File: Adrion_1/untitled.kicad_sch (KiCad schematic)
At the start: 3 parts, among them J6 M20-7821546, J7 M20-7821546, U6 NUCLEO-G431KB

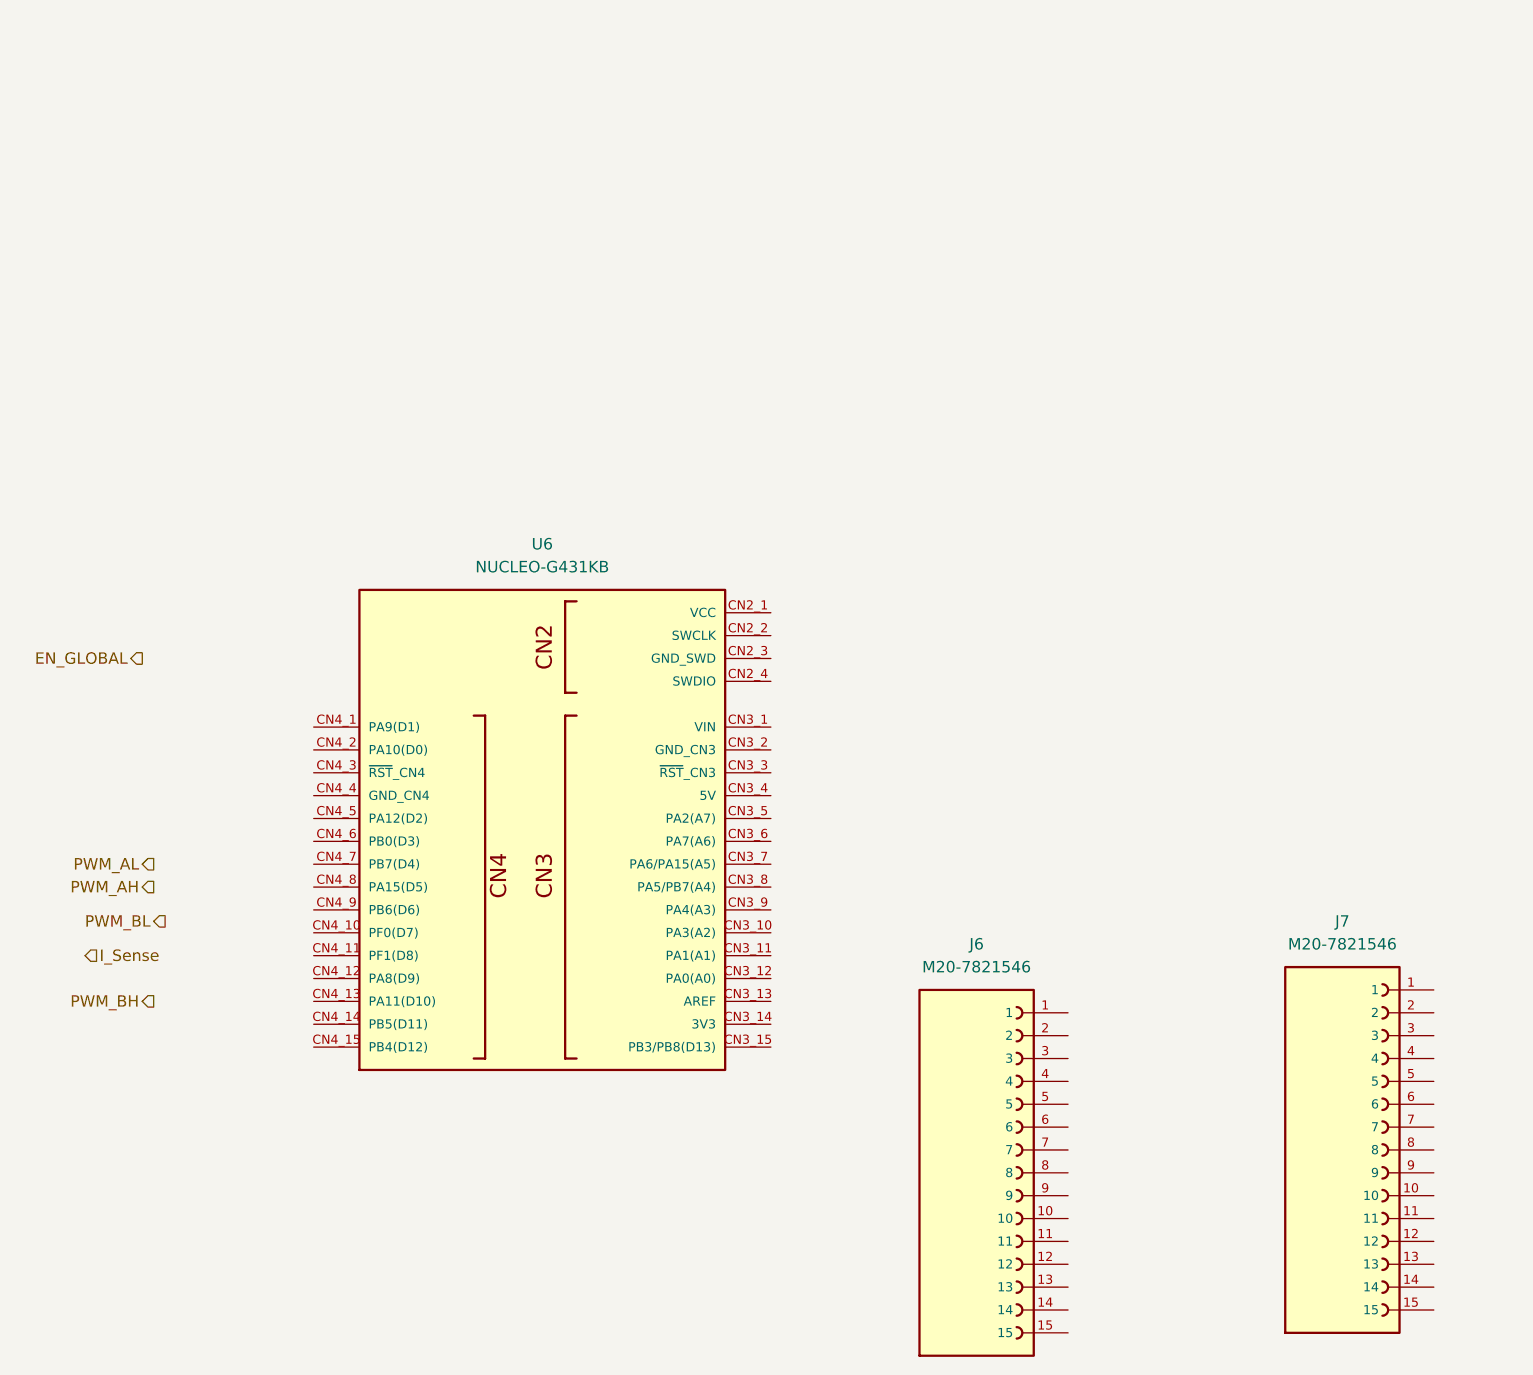
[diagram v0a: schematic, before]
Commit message: Mamita he empezado el layout. Vaya show
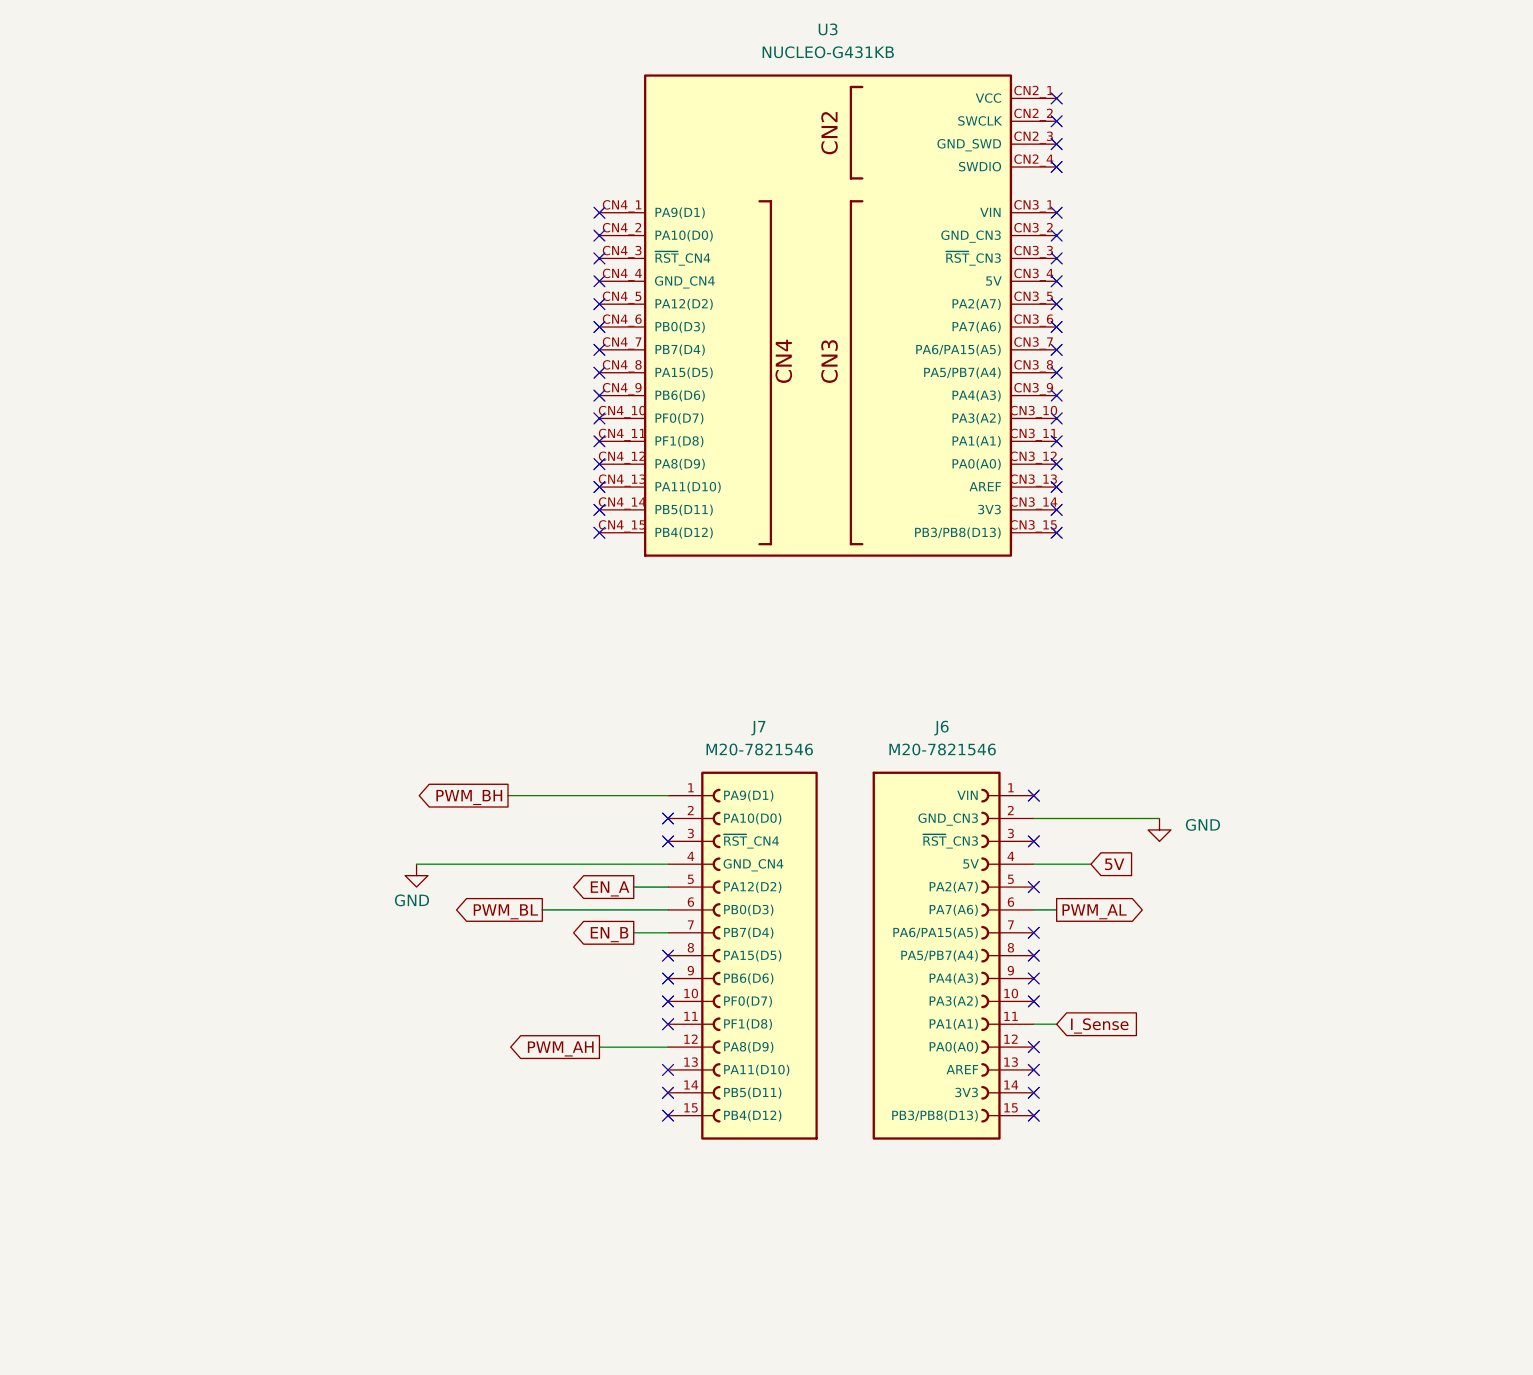
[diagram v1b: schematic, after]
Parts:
- removed U6: NUCLEO-G431KB, NUCLEO-G431KB:MODULE_NUCLEO-G431KB, symbol NUCLEO-G431KB:NUCLEO-G431KB
- added U3: NUCLEO-G431KB, MODULE_NUCLEO-G431KB:MODULE_NUCLEO-G431KB, symbol NUCLEO-G431KB:NUCLEO-G431KB
- J6, J7: footprint M20-7821546:HARWIN_M20-7821546 -> HARWIN_M20-7821546:HARWIN_M20-7821546
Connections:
- net I_Sense: now also J6.11 (PA1(A1))
- net PWM_AH: now also J7.12 (PA8(D9))
- net PWM_AL: now also J6.6 (PA7(A6))
- net PWM_BH: now also J7.1 (PA9(D1))
- net PWM_BL: now also J7.6 (PB0(D3))
- net GND: now reaches J7.4 (GND_CN4)
- net GND: now also J6.2 (GND_CN3)
- net EN_A: now reaches J7.5 (PA12(D2))
- net EN_B: now reaches J7.7 (PB7(D4))
- net 5V: now reaches J6.4 (5V)
- no-connect marks 0 -> 54
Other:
- moved on the sheet: J6, J7

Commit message: FirstPrototype
First Prototype sent
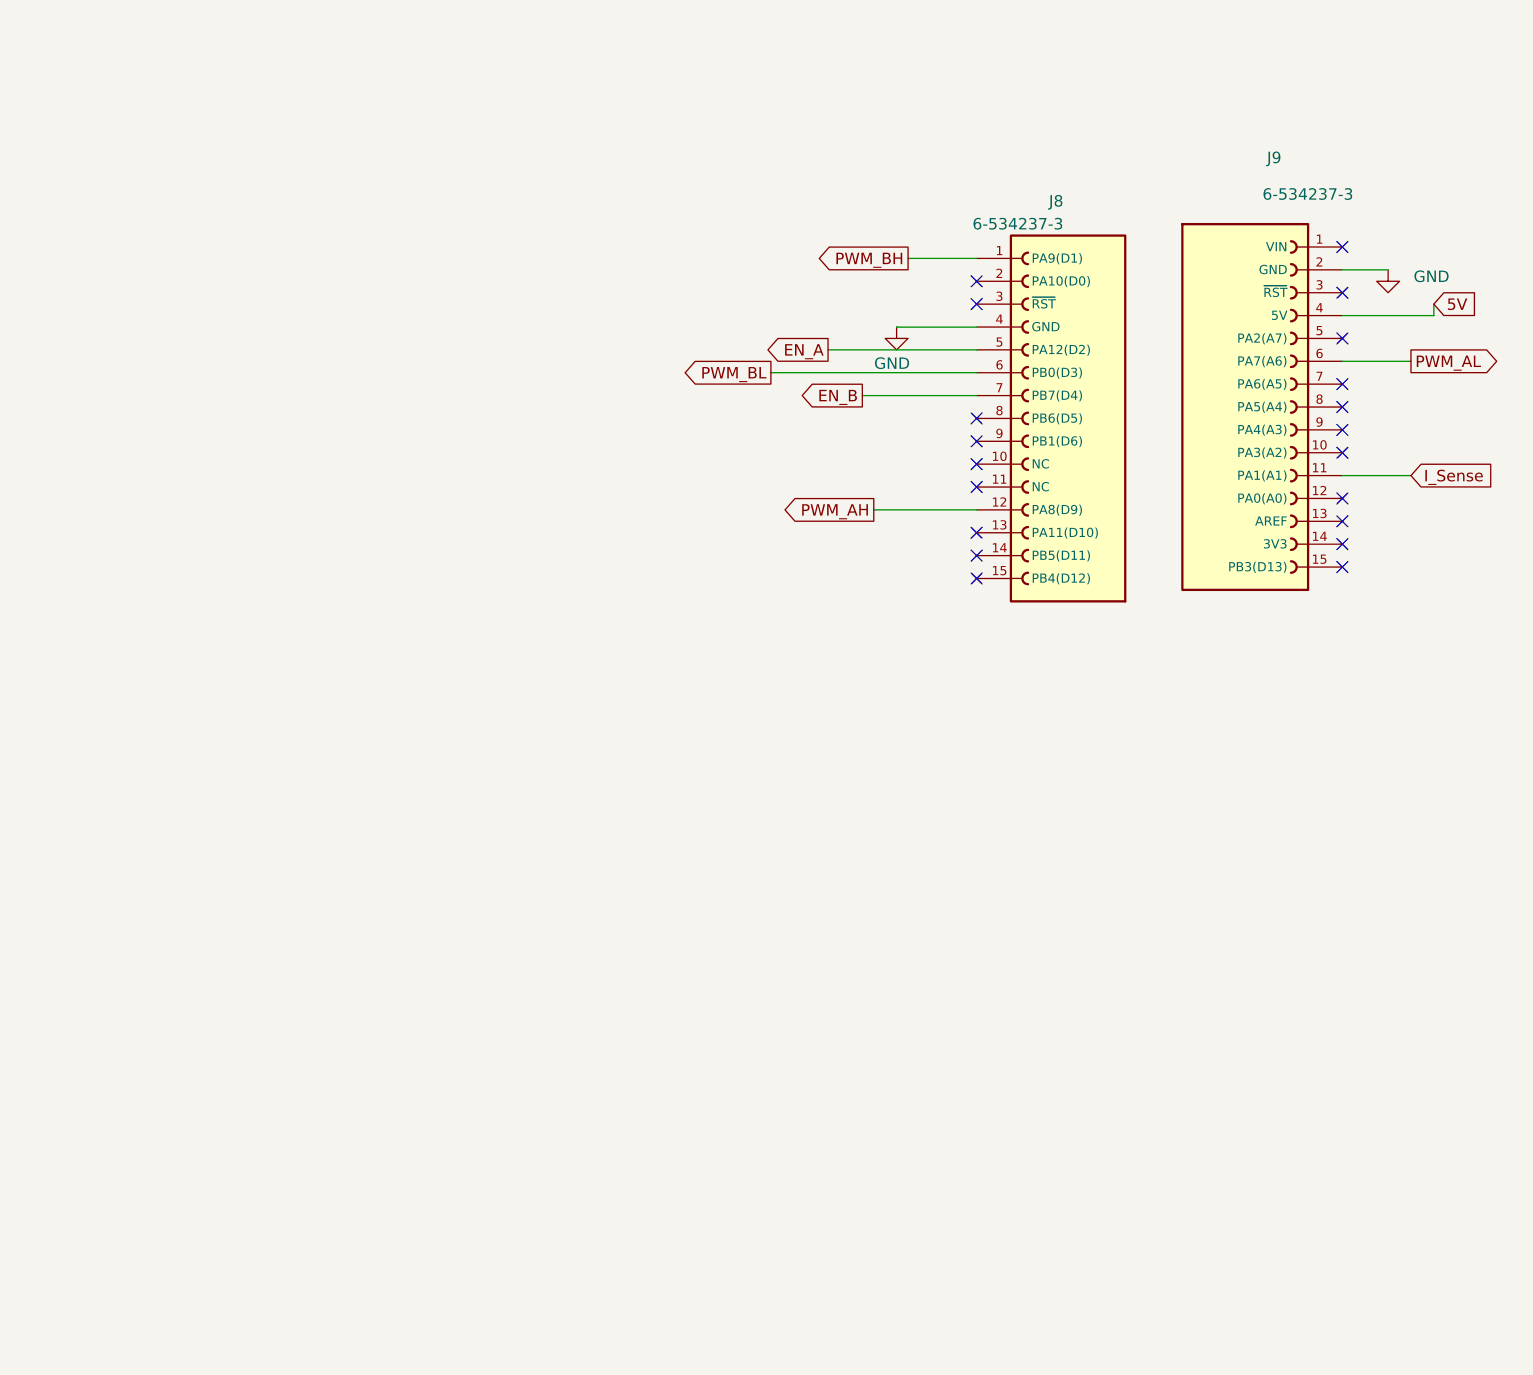
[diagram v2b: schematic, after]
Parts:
- removed J6, J7: M20-7821546, HARWIN_M20-7821546:HARWIN_M20-7821546, symbol M20-7821546:M20-7821546
- removed U3: NUCLEO-G431KB, MODULE_NUCLEO-G431KB:MODULE_NUCLEO-G431KB, symbol NUCLEO-G431KB:NUCLEO-G431KB
- added J8, J9: 6-534237-3, TE_6-534237-3:TE_6-534237-3, symbol 6-534237-3:6-534237-3
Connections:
- net 5V: now also J9.4 (5V)
- net EN_A: now also J8.5 (PA12(D2))
- net EN_B: now also J8.7 (PB7(D4))
- net GND: now also J8.4 (GND), J9.2 (GND)
- net I_Sense: now also J9.11 (PA1(A1))
- net PWM_AH: now also J8.12 (PA8(D9))
- net PWM_AL: now also J9.6 (PA7(A6))
- net PWM_BH: now also J8.1 (PA9(D1))
- net PWM_BL: now also J8.6 (PB0(D3))
- no-connect marks 54 -> 20
